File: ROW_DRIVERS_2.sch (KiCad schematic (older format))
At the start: 36 parts, among them Q120 DMG6602, Q121 DMG6602, Q122 SSM3K35AMFV, Q123 SSM3K35AMFV, Q124 SSM3K35AMFV, Q125 SSM3K35AMFV, Q126 DMG6602, Q127 DMG6602, Q128 SSM3K35AMFV, Q129 SSM3K35AMFV, Q130 SSM3K35AMFV, Q131 SSM3K35AMFV

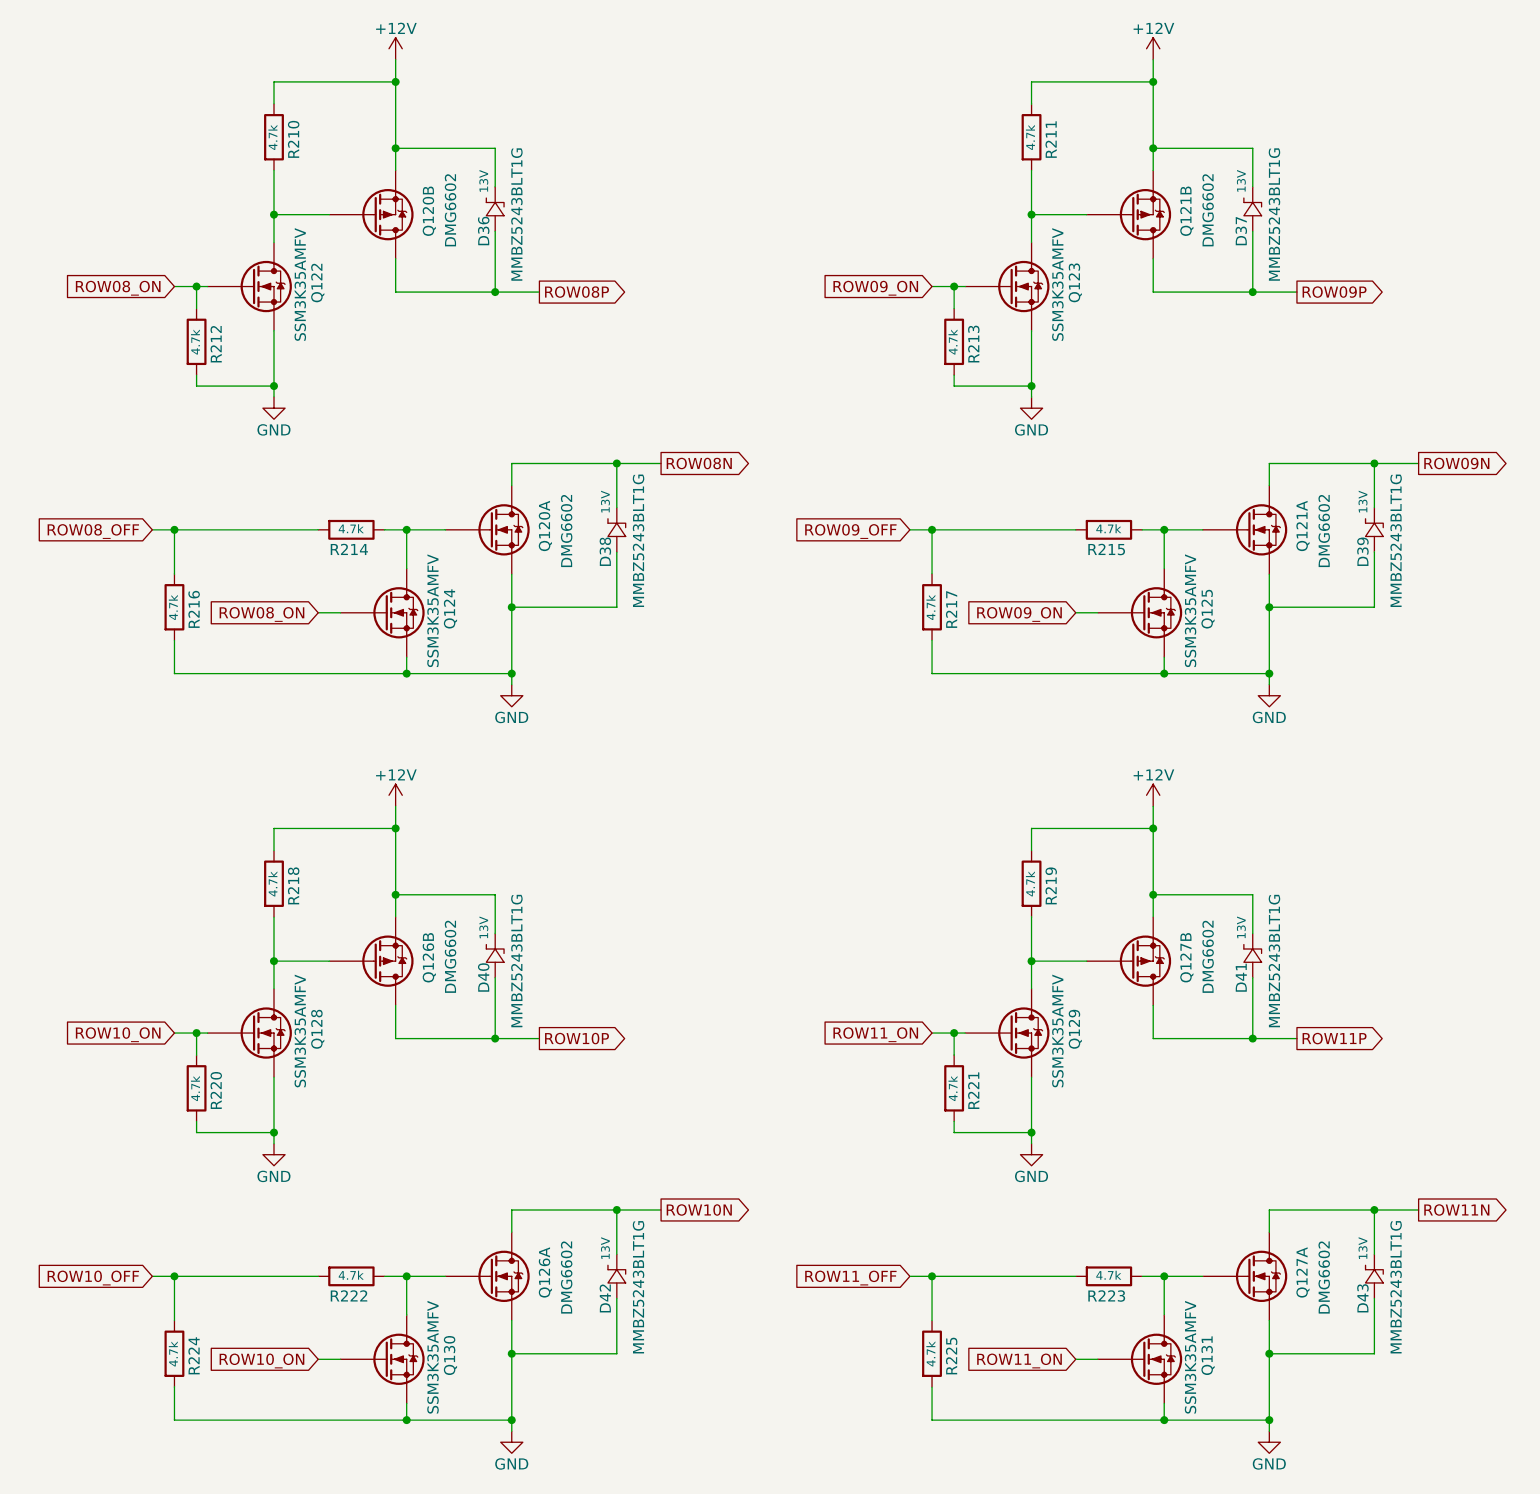
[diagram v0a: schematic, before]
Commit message: automated commit
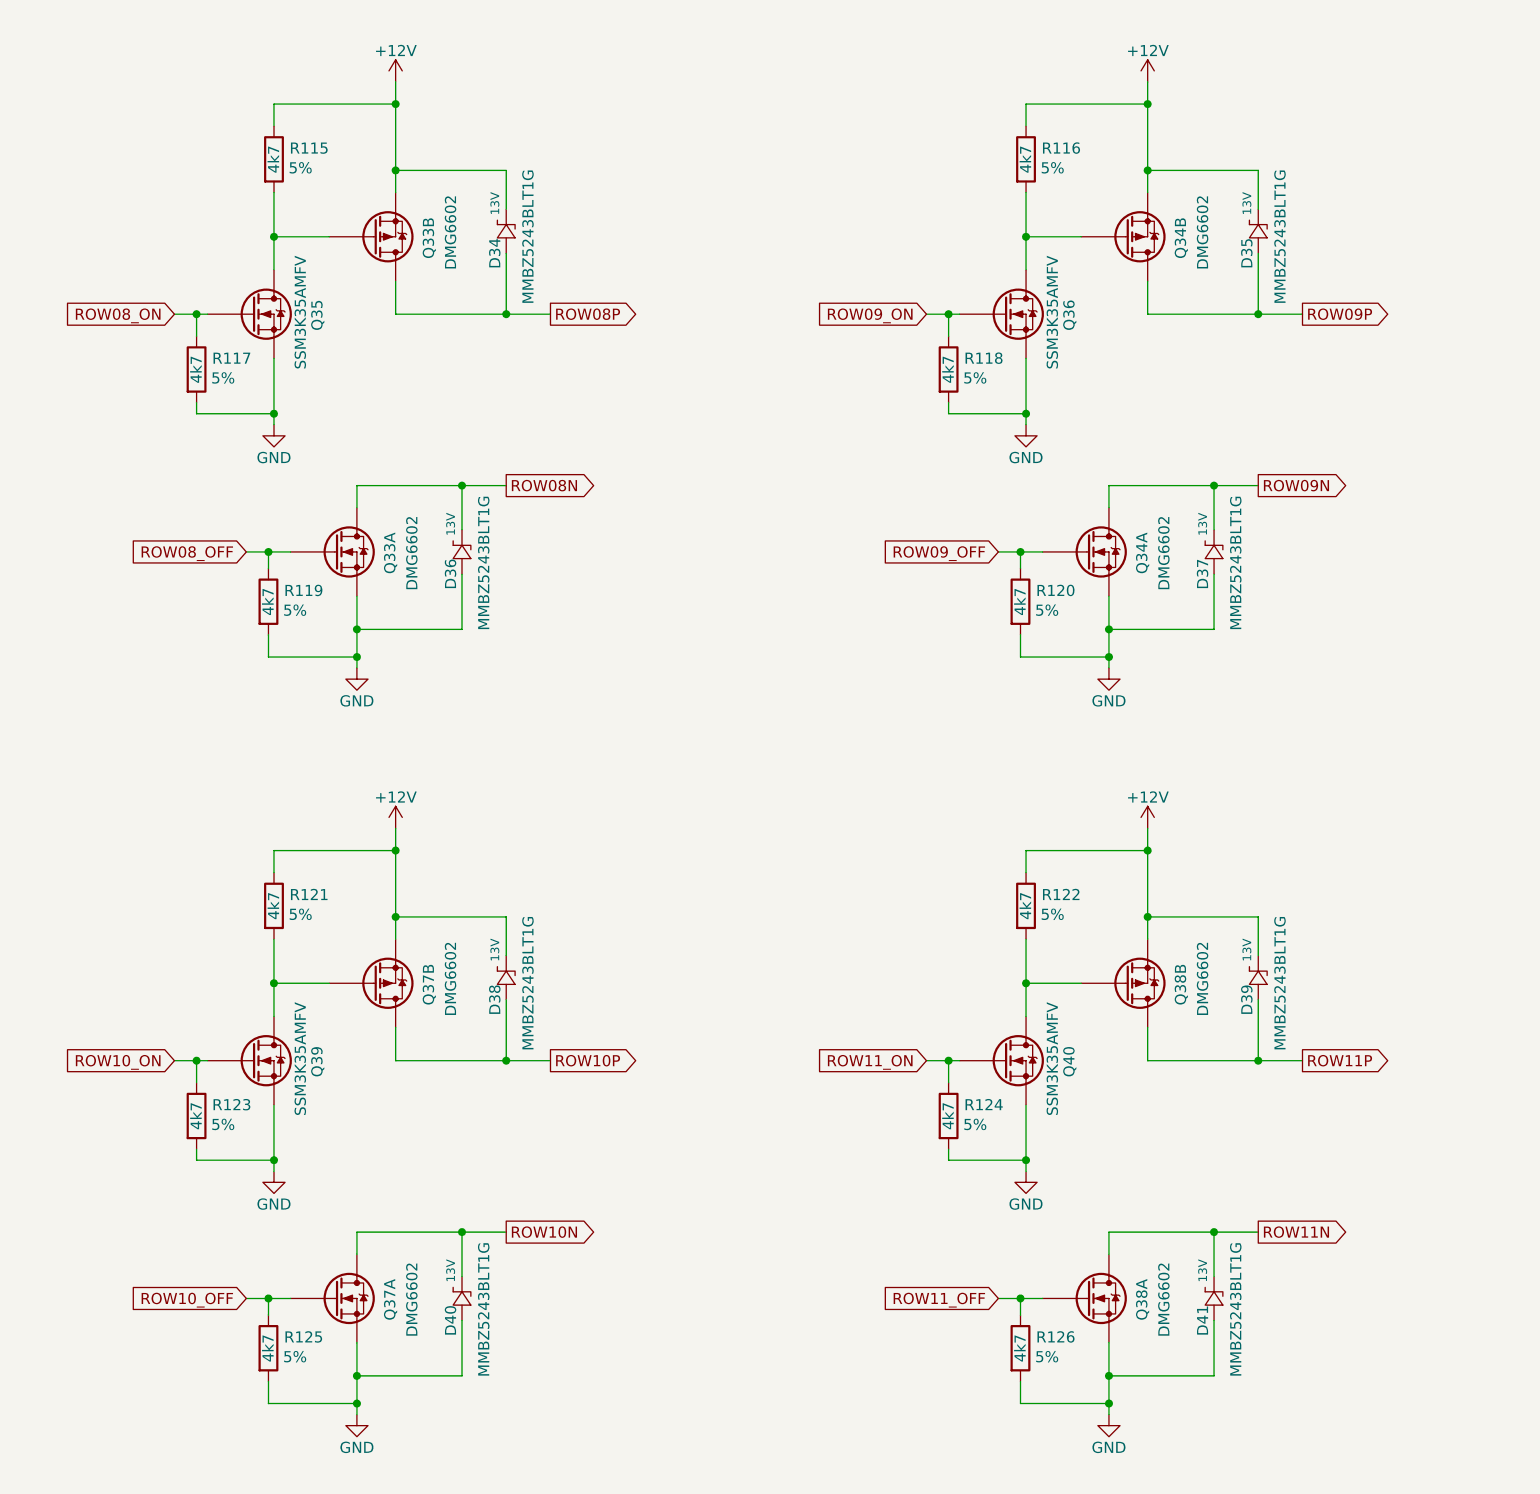
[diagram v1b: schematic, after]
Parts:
- removed D42, D43: MMBZ5243BLT1G, symbol custom:MMBZ5243BLT1G
- removed Q120, Q121, Q126, Q127: DMG6602, Package_TO_SOT_SMD:TSOT-23-6, symbol custom:DMG6602
- removed Q122, Q123, Q124, Q125, Q128, Q129, Q130, Q131: SSM3K35AMFV, symbol custom:SSM3K35AMFV
- removed R210, R211, R212, R213, R214, R215, R216, R217, R218, R219, R220, R221, R222, R223, R224, R225: CRG0603F4K7, Resistor_SMD:R_0603_1608Metric, symbol custom:CRG0603F4K7
- added D34, D35: MMBZ5243BLT1G, symbol custom:MMBZ5243BLT1G
- added Q33, Q34, Q37, Q38: DMG6602, Package_TO_SOT_SMD:TSOT-23-6, symbol custom:DMG6602
- added Q35, Q36, Q39, Q40: SSM3K35AMFV, symbol custom:SSM3K35AMFV
- added R115, R116, R117, R118, R119, R120, R121, R122, R123, R124, R125, R126: CRG0603F4K7, Resistor_SMD:R_0603_1608Metric, symbol custom:CRG0603F4K7
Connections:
- net +12V: now also D38.1 (K), D39.1 (K), D34.1 (K), D35.1 (K), Q33.2 (S), Q34.2 (S), Q37.2 (S), Q38.2 (S), R115.1, R116.1, R121.1, R122.1; no longer D36.1 (K), D37.1 (K), D40.1 (K), D41.1 (K)
- net GND: now also D36.2 (A), D37.2 (A), D40.2 (A), D41.2 (A), Q33.5 (S), Q34.5 (S), Q35.2 (S), Q36.2 (S), Q37.5 (S), Q38.5 (S), Q39.2 (S), Q40.2 (S), R117.2, R118.2, R119.2, R120.2, R123.2, R124.2, R125.2, R126.2; no longer D38.2 (A), D39.2 (A)
- net ROW08N: now also D36.1 (K), Q33.6 (D); no longer D38.1 (K)
- net ROW08P: now also D34.2 (A), Q33.4 (D); no longer D36.2 (A)
- net ROW08_OFF: now also Q33.1 (G), R119.1
- net ROW08_ON: now also Q35.1 (G), R117.1
- net ROW09N: now also D37.1 (K), Q34.6 (D); no longer D39.1 (K)
- net ROW09P: now also D35.2 (A), Q34.4 (D); no longer D37.2 (A)
- net ROW09_OFF: now also Q34.1 (G), R120.1
- net ROW09_ON: now also Q36.1 (G), R118.1
- net ROW10N: now also D40.1 (K), Q37.6 (D)
- net ROW10P: now also D38.2 (A), Q37.4 (D); no longer D40.2 (A)
- net ROW10_OFF: now also Q37.1 (G), R125.1
- net ROW10_ON: now also Q39.1 (G), R123.1
- net ROW11N: now also D41.1 (K), Q38.6 (D)
- net ROW11P: now also D39.2 (A), Q38.4 (D); no longer D41.2 (A)
- net ROW11_OFF: now also Q38.1 (G), R126.1
- net ROW11_ON: now also Q40.1 (G), R124.1
- new net: Q34.3 (G), Q36.3 (D), R116.2
- new net: Q38.3 (G), Q40.3 (D), R122.2
- new net: Q37.3 (G), Q39.3 (D), R121.2
- new net: Q33.3 (G), Q35.3 (D), R115.2
